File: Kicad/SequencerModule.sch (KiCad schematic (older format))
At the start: 13 parts, among them U1 L78L05_SOT89, U2 MCP4822

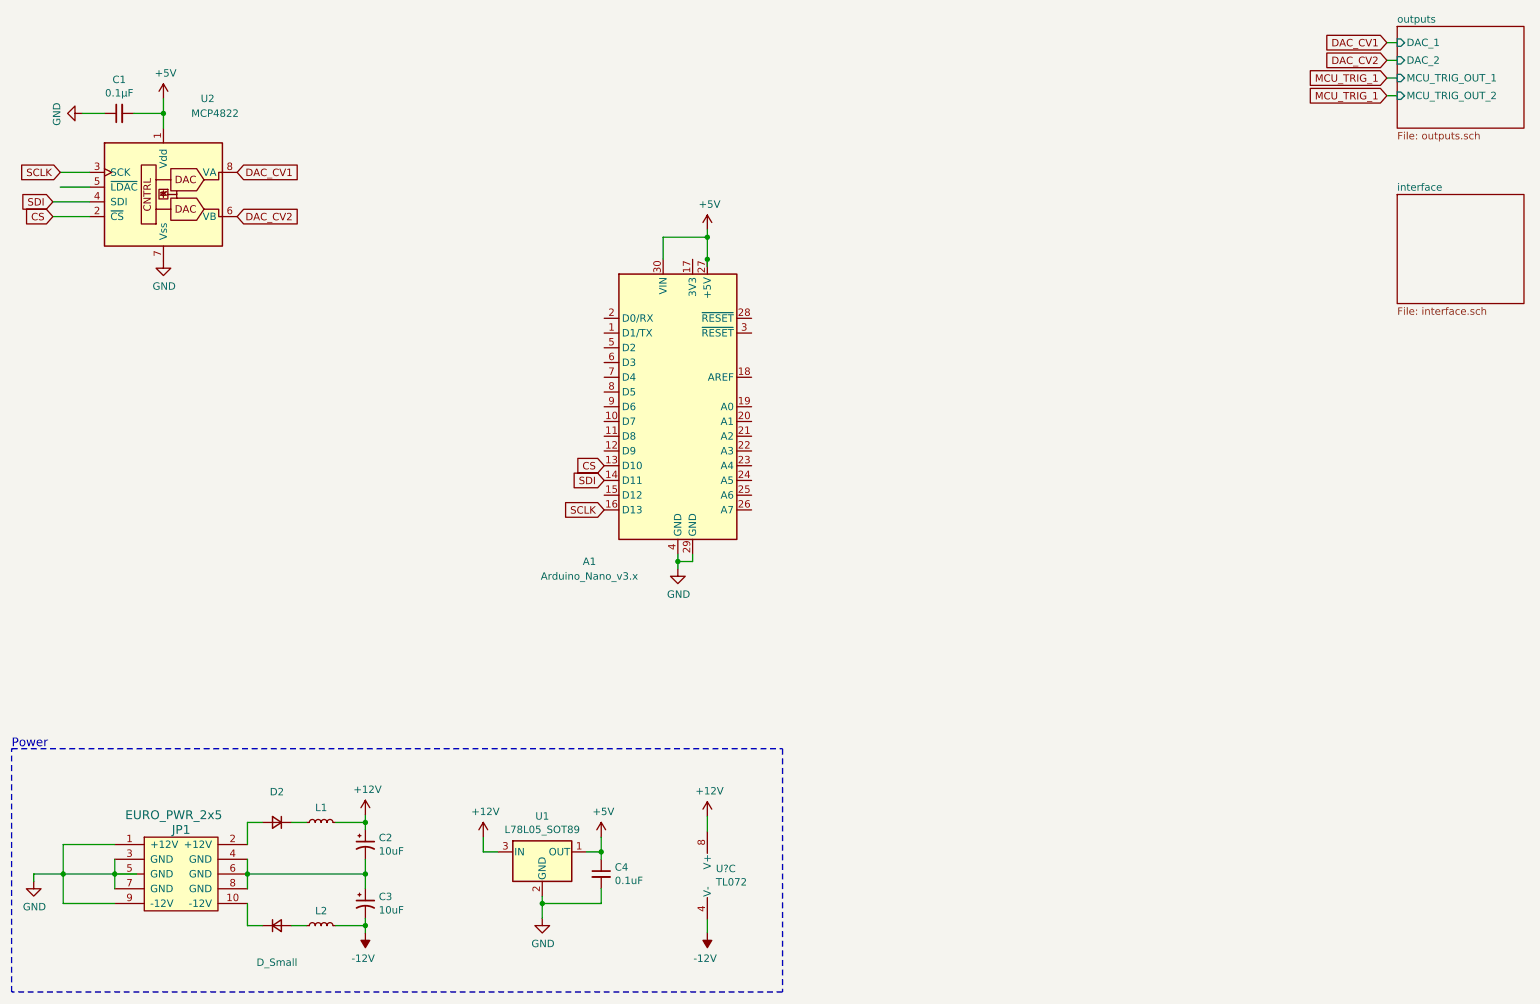
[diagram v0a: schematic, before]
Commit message: making progress on interface
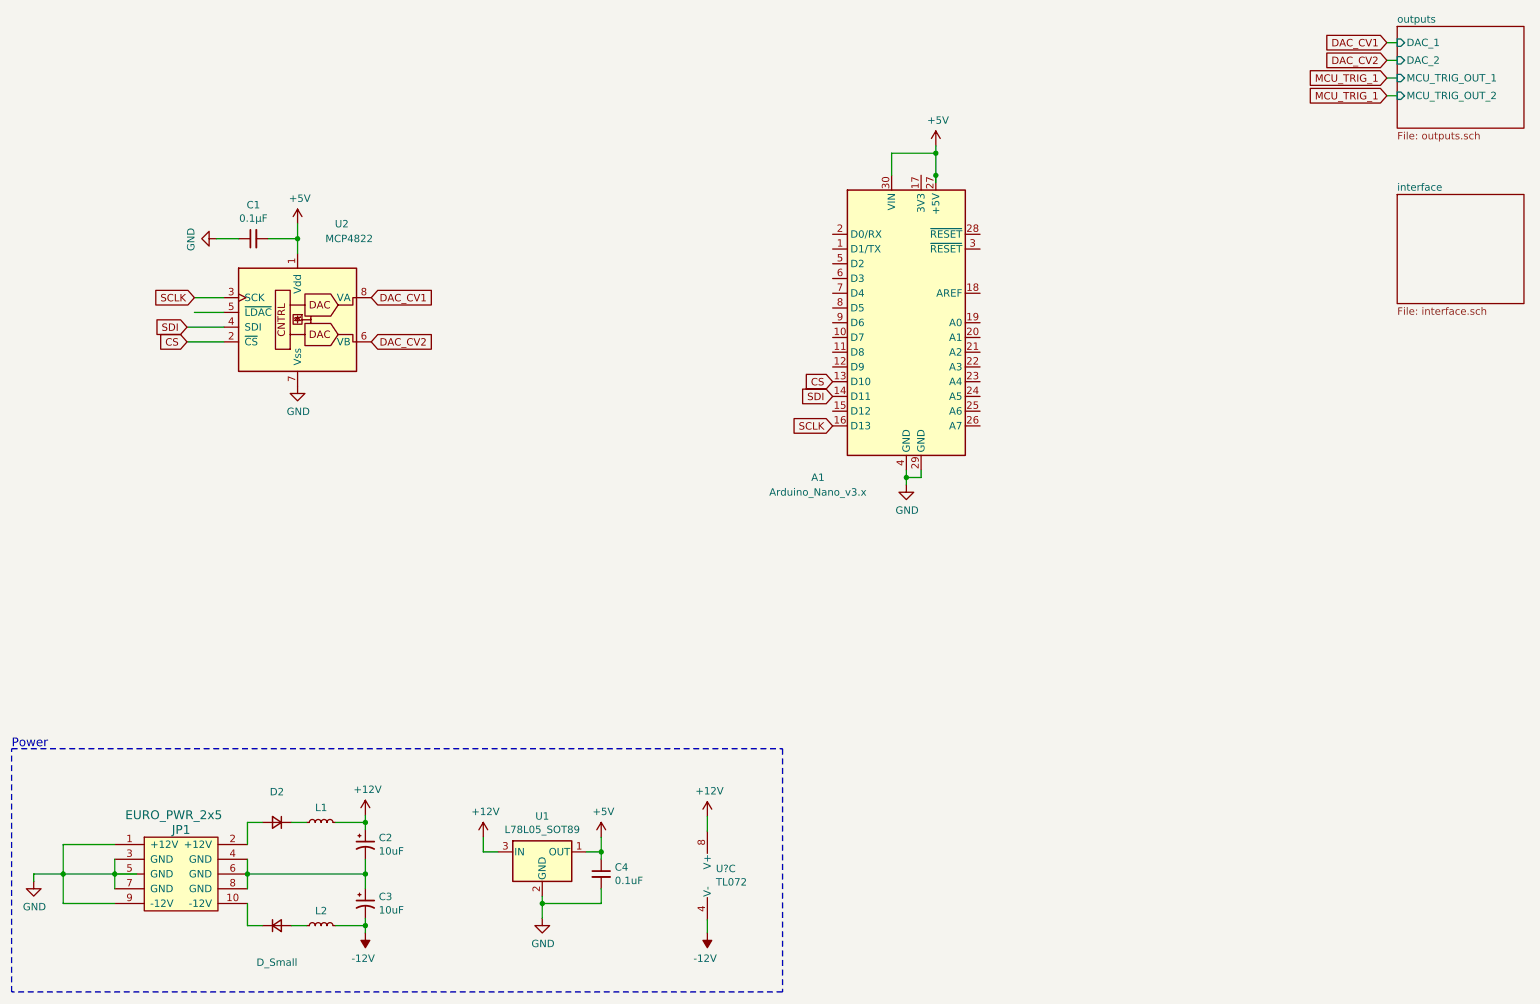
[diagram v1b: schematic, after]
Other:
- moved on the sheet: A1, C1, U2
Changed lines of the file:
@@
 L Analog_DAC:MCP4822 U2
 U 1 1 5FAC40C6
-P 1880 2090
-F 0 "U2" H 2180 2690 50  0000 C CNN
-F 1 "MCP4822" H 2230 2590 50  0000 C CNN
-F 2 "" H 2680 1790 50  0001 C CNN
-F 3 "http://ww1.microchip.com/downloads/en/DeviceDoc/20002249B.pdf" H 2680 1790 50  0001 C CNN
-	1    1880 2090
+P 2790 2940
+F 0 "U2" H 3090 3540 50  0000 C CNN
+F 1 "MCP4822" H 3140 3440 50  0000 C CNN
+F 2 "" H 3590 2640 50  0001 C CNN
+F 3 "http://ww1.microchip.com/downloads/en/DeviceDoc/20002249B.pdf" H 3590 2640 50  0001 C CNN
+	1    2790 2940
 	1    0    0    -1
 $EndComp
@@
 L power:GND #PWR0101
 U 1 1 5FAC5967
-P 1880 2590
-F 0 "#PWR0101" H 1880 2340 50  0001 C CNN
-F 1 "GND" H 1885 2417 50  0000 C CNN
-F 2 "" H 1880 2590 50  0001 C CNN
-F 3 "" H 1880 2590 50  0001 C CNN
-	1    1880 2590
+P 2790 3440
+F 0 "#PWR0101" H 2790 3190 50  0001 C CNN
+F 1 "GND" H 2795 3267 50  0000 C CNN
+F 2 "" H 2790 3440 50  0001 C CNN
+F 3 "" H 2790 3440 50  0001 C CNN
+	1    2790 3440
 	1    0    0    -1
 $EndComp
@@
 L Device:C_Small C1
 U 1 1 5FAC8AF5
-P 1580 1590
-F 0 "C1" V 1809 1590 50  0000 C CNN
-F 1 "0.1μF" V 1718 1590 50  0000 C CNN
-F 2 "" H 1580 1590 50  0001 C CNN
-F 3 "~" H 1580 1590 50  0001 C CNN
-	1    1580 1590
+P 2490 2440
+F 0 "C1" V 2719 2440 50  0000 C CNN
+F 1 "0.1μF" V 2628 2440 50  0000 C CNN
+F 2 "" H 2490 2440 50  0001 C CNN
+F 3 "~" H 2490 2440 50  0001 C CNN
+	1    2490 2440
 	0    -1   -1   0
 $EndComp
 Wire Wire Line
-	1880 1490 1880 1590
-Wire Wire Line
-	1680 1590 1880 1590
-Connection ~ 1880 1590
-Wire Wire Line
-	1880 1590 1880 1690
+	2790 2340 2790 2440
+Wire Wire Line
+	2590 2440 2790 2440
+Connection ~ 2790 2440
+Wire Wire Line
+	2790 2440 2790 2540
 $Comp
 L power:GND #PWR0102
 U 1 1 5FAC9D1B
-P 1330 1590
-F 0 "#PWR0102" H 1330 1340 50  0001 C CNN
-F 1 "GND" H 1335 1417 50  0000 C CNN
-F 2 "" H 1330 1590 50  0001 C CNN
-F 3 "" H 1330 1590 50  0001 C CNN
-	1    1330 1590
+P 2240 2440
+F 0 "#PWR0102" H 2240 2190 50  0001 C CNN
+F 1 "GND" H 2245 2267 50  0000 C CNN
+F 2 "" H 2240 2440 50  0001 C CNN
+F 3 "" H 2240 2440 50  0001 C CNN
+	1    2240 2440
 	0    1    1    0
 $EndComp
 Wire Wire Line
-	1330 1590 1480 1590
-Text GLabel 1180 1990 0    50   Input ~ 0
+	2240 2440 2390 2440
+Text GLabel 2090 2840 0    50   Input ~ 0
 SCLK
-Text GLabel 1130 2290 0    50   Input ~ 0
+Text GLabel 2040 3140 0    50   Input ~ 0
 CS
-Text GLabel 2380 1990 2    50   Input ~ 0
+Text GLabel 3290 2840 2    50   Input ~ 0
 DAC_CV1
-Text GLabel 2380 2290 2    50   Input ~ 0
+Text GLabel 3290 3140 2    50   Input ~ 0
 DAC_CV2
 Wire Wire Line
-	1180 1990 1380 1990
-Wire Wire Line
-	1180 2090 1380 2090
-Wire Wire Line
-	1130 2190 1380 2190
-Wire Wire Line
-	1130 2290 1380 2290
+	2090 2840 2290 2840
+Wire Wire Line
+	2090 2940 2290 2940
+Wire Wire Line
+	2040 3040 2290 3040
+Wire Wire Line
+	2040 3140 2290 3140
 $Comp
 L MCU_Module:Arduino_Nano_v3.x A1
 U 1 1 5FAD0791
-P 5370 3580
-F 0 "A1" H 4770 2530 50  0000 C CNN
-F 1 "Arduino_Nano_v3.x" H 4770 2430 50  0000 C CNN
-F 2 "Module:Arduino_Nano" H 5370 3580 50  0001 C CIN
-F 3 "http://www.mouser.com/pdfdocs/Gravitech_Arduino_Nano3_0.pdf" H 5370 3580 50  0001 C CNN
-	1    5370 3580
+P 6920 3010
+F 0 "A1" H 6320 1960 50  0000 C CNN
+F 1 "Arduino_Nano_v3.x" H 6320 1860 50  0000 C CNN
+F 2 "Module:Arduino_Nano" H 6920 3010 50  0001 C CIN
+F 3 "http://www.mouser.com/pdfdocs/Gravitech_Arduino_Nano3_0.pdf" H 6920 3010 50  0001 C CNN
+	1    6920 3010
 	1    0    0    -1
 $EndComp
@@
 L power:GND #PWR0103
 U 1 1 5FAD2D29
-P 5370 4680
-F 0 "#PWR0103" H 5370 4430 50  0001 C CNN
-F 1 "GND" H 5375 4507 50  0000 C CNN
-F 2 "" H 5370 4680 50  0001 C CNN
-F 3 "" H 5370 4680 50  0001 C CNN
-	1    5370 4680
-	1    0    0    -1
-$EndComp
-Wire Wire Line
-	5370 4580 5370 4630
-Wire Wire Line
-	5470 4580 5470 4630
-Wire Wire Line
-	5470 4630 5370 4630
-Connection ~ 5370 4630
-Wire Wire Line
-	5370 4630 5370 4680
-Text GLabel 4870 4080 0    50   Input ~ 0
+P 6920 4110
+F 0 "#PWR0103" H 6920 3860 50  0001 C CNN
+F 1 "GND" H 6925 3937 50  0000 C CNN
+F 2 "" H 6920 4110 50  0001 C CNN
+F 3 "" H 6920 4110 50  0001 C CNN
+	1    6920 4110
+	1    0    0    -1
+$EndComp
+Wire Wire Line
+	6920 4010 6920 4060
+Wire Wire Line
+	7020 4010 7020 4060
+Wire Wire Line
+	7020 4060 6920 4060
+Connection ~ 6920 4060
+Wire Wire Line
+	6920 4060 6920 4110
+Text GLabel 6420 3510 0    50   Input ~ 0
 SDI
-Text GLabel 1130 2190 0    50   Input ~ 0
+Text GLabel 2040 3040 0    50   Input ~ 0
 SDI
-Text GLabel 4870 4280 0    50   Input ~ 0
+Text GLabel 6420 3710 0    50   Input ~ 0
 SCLK
 $Comp
@@
 L power:+5V #PWR0110
 U 1 1 5FB4B6EF
-P 1880 1490
-F 0 "#PWR0110" H 1880 1340 50  0001 C CNN
-F 1 "+5V" H 1895 1663 50  0000 C CNN
-F 2 "" H 1880 1490 50  0001 C CNN
-F 3 "" H 1880 1490 50  0001 C CNN
-	1    1880 1490
+P 2790 2340
+F 0 "#PWR0110" H 2790 2190 50  0001 C CNN
+F 1 "+5V" H 2805 2513 50  0000 C CNN
+F 2 "" H 2790 2340 50  0001 C CNN
+F 3 "" H 2790 2340 50  0001 C CNN
+	1    2790 2340
 	1    0    0    -1
 $EndComp
@@
 L power:+5V #PWR0113
 U 1 1 5FB529CE
-P 5570 2380
-F 0 "#PWR0113" H 5570 2230 50  0001 C CNN
-F 1 "+5V" H 5585 2553 50  0000 C CNN
-F 2 "" H 5570 2380 50  0001 C CNN
-F 3 "" H 5570 2380 50  0001 C CNN
-	1    5570 2380
-	1    0    0    -1
-$EndComp
-Wire Wire Line
-	5570 2630 5570 2580
-Wire Wire Line
-	5570 2380 5570 2430
-Connection ~ 5570 2580
-Wire Wire Line
-	5270 2580 5270 2430
-Wire Wire Line
-	5270 2430 5570 2430
-Connection ~ 5570 2430
-Wire Wire Line
-	5570 2430 5570 2580
-Text GLabel 4870 3980 0    50   Input ~ 0
+P 7120 1810
+F 0 "#PWR0113" H 7120 1660 50  0001 C CNN
+F 1 "+5V" H 7135 1983 50  0000 C CNN
+F 2 "" H 7120 1810 50  0001 C CNN
+F 3 "" H 7120 1810 50  0001 C CNN
+	1    7120 1810
+	1    0    0    -1
+$EndComp
+Wire Wire Line
+	7120 2060 7120 2010
+Wire Wire Line
+	7120 1810 7120 1860
+Connection ~ 7120 2010
+Wire Wire Line
+	6820 2010 6820 1860
+Wire Wire Line
+	6820 1860 7120 1860
+Connection ~ 7120 1860
+Wire Wire Line
+	7120 1860 7120 2010
+Text GLabel 6420 3410 0    50   Input ~ 0
 CS
 $Comp
